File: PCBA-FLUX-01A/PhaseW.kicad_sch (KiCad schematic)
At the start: 60 parts, among them Q12 IPT015N10N5, Q13 IPT015N10N5, Q14 IPT015N10N5, Q15 IPT015N10N5, Q16 BC817, U10 TLV9001, U8 INA240A2DR, U9 UCC27211AQDDARQ1

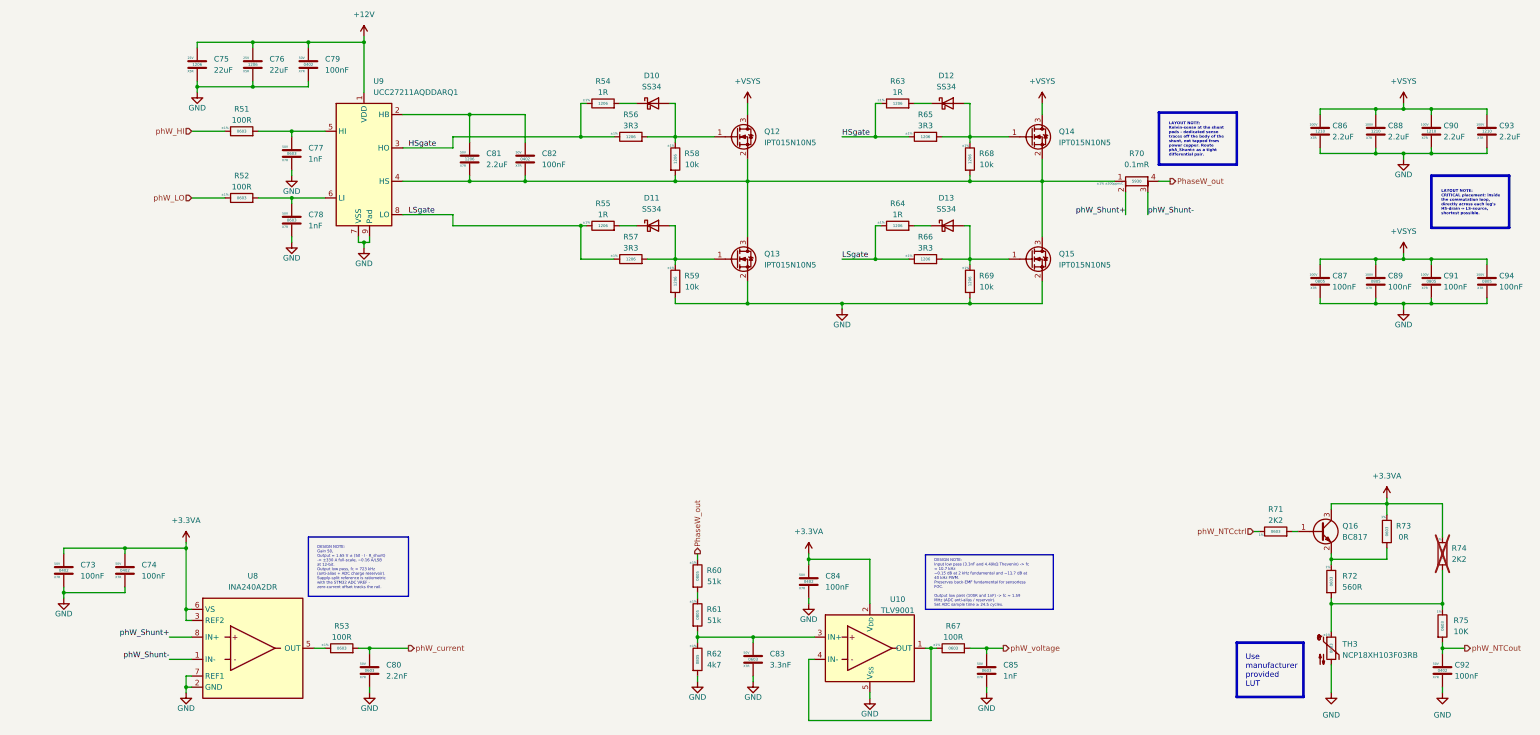
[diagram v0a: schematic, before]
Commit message: Changes were made
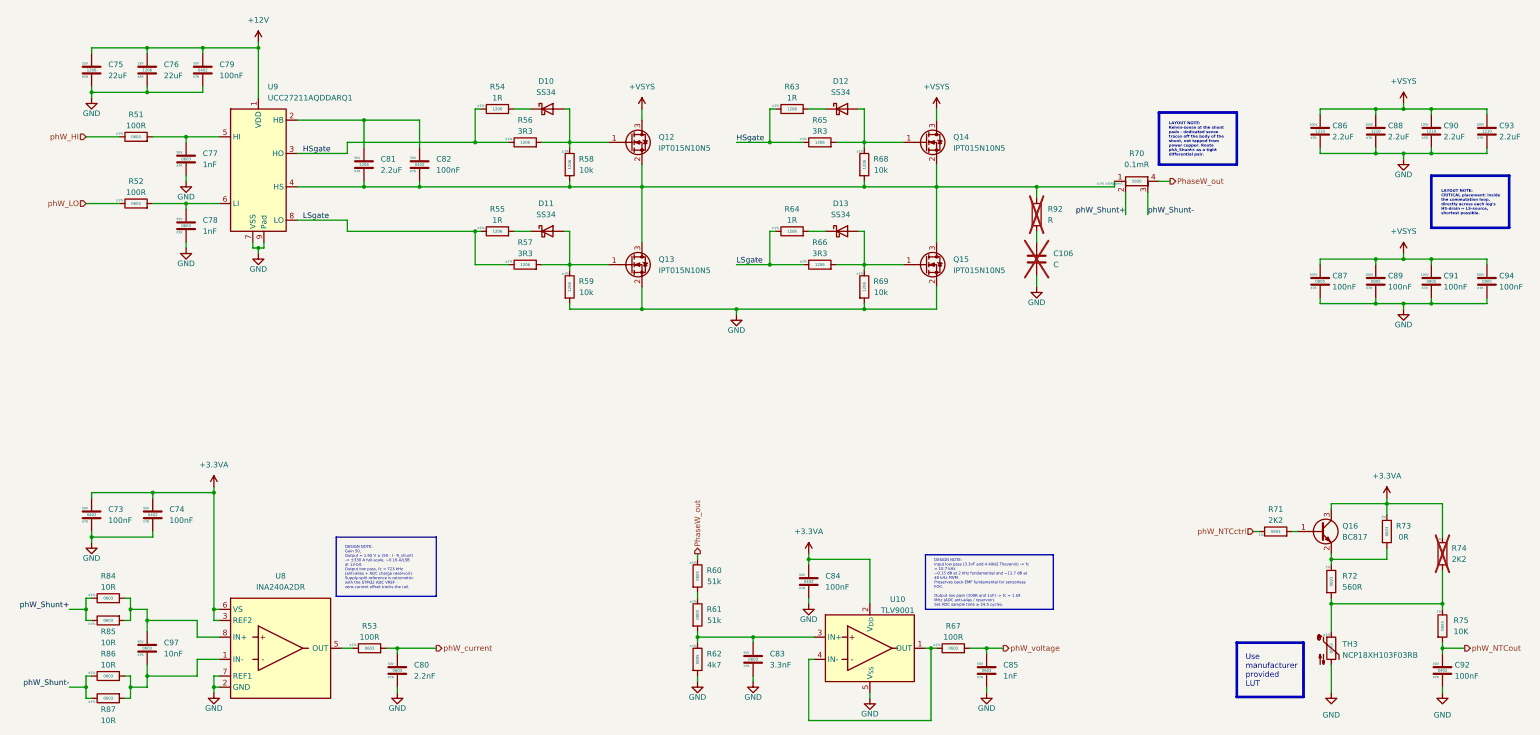
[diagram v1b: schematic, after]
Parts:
- added C106: C, Capacitor_THT:C_Rect_L9.0mm_W6.4mm_P7.50mm_MKT, symbol Device:C
- added C97: 10nF, Capacitor_SMD:C_0603_1608Metric, symbol Device:C
- added R84, R85, R86, R87: 10R, Resistor_SMD:R_0805_2012Metric, symbol Device:R
- added R92: R, Resistor_SMD:R_1218_3246Metric, symbol Device:R
- R51, R52, R53, R67: footprint Resistor_SMD:R_0805_2012Metric -> Resistor_SMD:R_0603_1608Metric
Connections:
- net GND: now also C106.2
- net phW_Shunt+: now also R84.1, R85.1; no longer U8.8 (IN+)
- net phW_Shunt-: now also R86.1, R87.1; no longer U8.1 (IN-)
- net at C81.2, C82.2, Q12.2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: now also R92.1
- new net: C97.2, R86.2, R87.2, U8.1 (IN-)
- new net: C97.1, R84.2, R85.2, U8.8 (IN+)
- new net: C106.1, R92.2
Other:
- moved on the sheet: C75, C76, C77, C78, C79, C80, C81, C82, D10, D11, D12, D13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
